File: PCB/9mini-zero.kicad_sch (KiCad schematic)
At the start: 16 parts

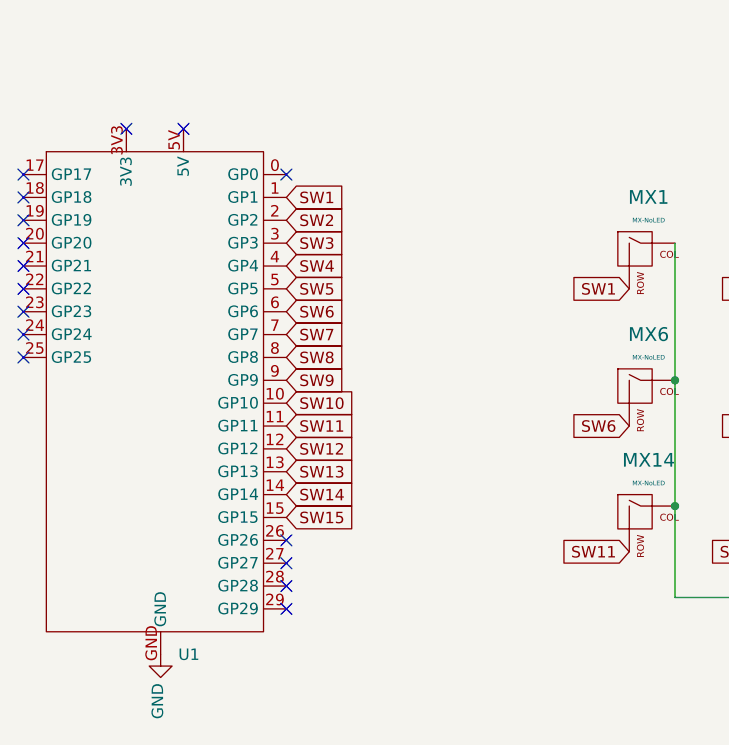
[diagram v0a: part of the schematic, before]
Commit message: board layout
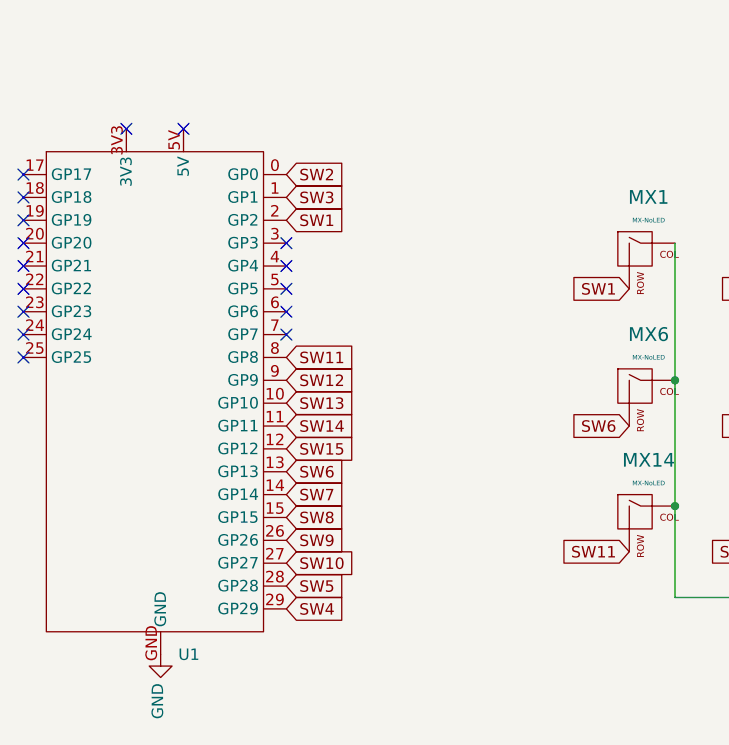
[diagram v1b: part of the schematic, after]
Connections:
- net SW1: now also U1.2 (GP2); no longer U1.1 (GP1)
- net SW10: now also U1.27 (GP27); no longer U1.10 (GP10)
- net SW11: now also U1.8 (GP8); no longer U1.11 (GP11)
- net SW12: now also U1.9 (GP9); no longer U1.12 (GP12)
- net SW13: now also U1.10 (GP10); no longer U1.13 (GP13)
- net SW14: now also U1.11 (GP11); no longer U1.14 (GP14)
- net SW15: now also U1.12 (GP12); no longer U1.15 (GP15)
- net SW2: now also U1.0 (GP0); no longer U1.2 (GP2)
- net SW3: now also U1.1 (GP1); no longer U1.3 (GP3)
- net SW4: now also U1.29 (GP29); no longer U1.4 (GP4)
- net SW5: now also U1.28 (GP28); no longer U1.5 (GP5)
- net SW6: now also U1.13 (GP13); no longer U1.6 (GP6)
- net SW7: now also U1.14 (GP14); no longer U1.7 (GP7)
- net SW8: now also U1.15 (GP15); no longer U1.8 (GP8)
- net SW9: now also U1.26 (GP26); no longer U1.9 (GP9)
